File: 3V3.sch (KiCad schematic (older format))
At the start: 1 part, among them SW4 SW_SP3T

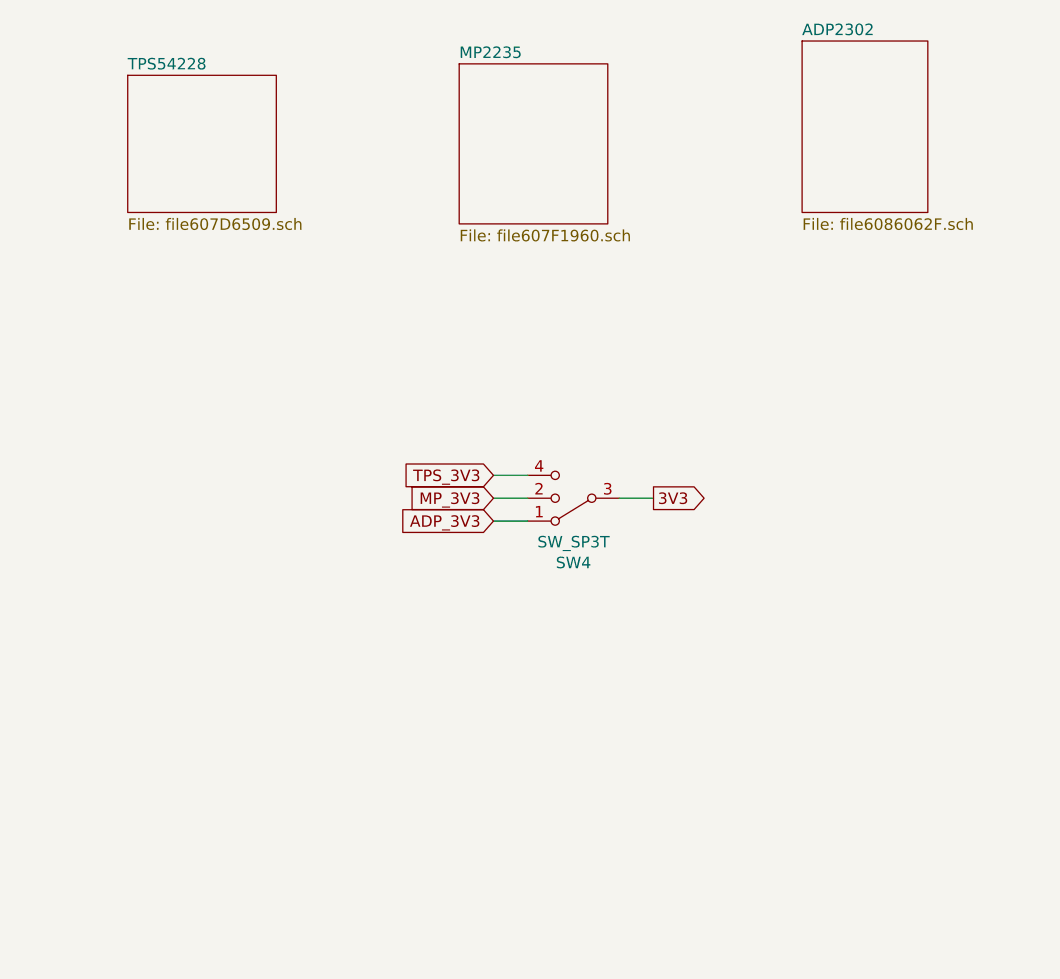
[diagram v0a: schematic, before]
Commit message: full schematic, version 1.0
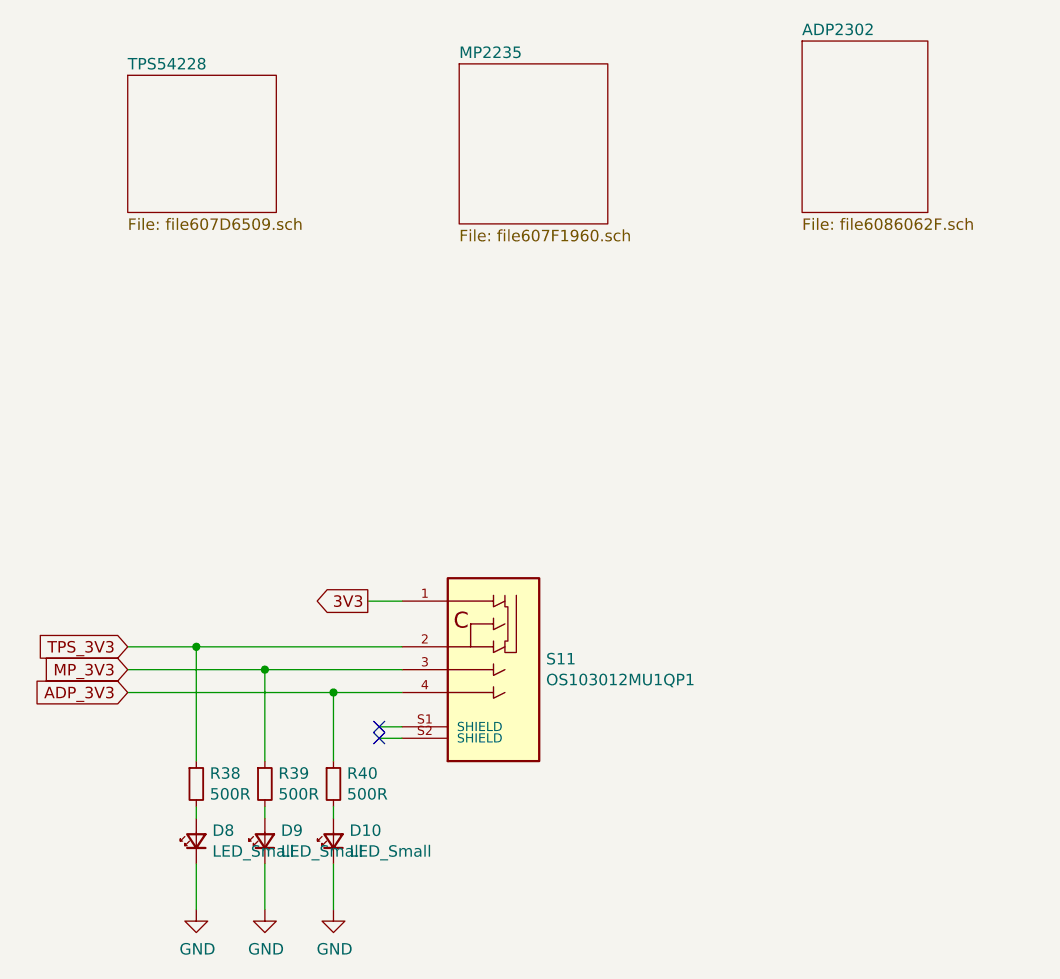
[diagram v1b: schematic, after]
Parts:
- removed SW4: SW_SP3T, symbol Switch:SW_SP3T
- added D10, D8, D9: LED_Small, Diode_SMD:D_0603_1608Metric_Pad1.05x0.95mm_HandSolder, symbol Device:LED_Small
- added R38, R39, R40: 500R, Resistor_SMD:R_0805_2012Metric_Pad1.20x1.40mm_HandSolder, symbol Device:R_Small
- added S11: OS103012MU1QP1, EIPP:SW_OS103012MU1QP1, symbol EIPP_LIBRARY:OS103012MU1QP1
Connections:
- net 3V3: now also S11.1
- net ADP_3V3: now also R40.1, S11.4
- net MP_3V3: now also R39.1, S11.3
- net TPS_3V3: now also R38.1, S11.2
- new net: D8.2 (A), R38.2
- new net: D9.2 (A), R39.2
- new net: D10.2 (A), R40.2
- new net GND: D10.1 (K), D8.1 (K), D9.1 (K)
- no-connect marks 0 -> 2
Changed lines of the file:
@@
 $Descr A4 11693 8268
 encoding utf-8
-Sheet 2 10
+Sheet 2 15
 Title ""
 Date ""
@@
 F1 "file6086062F.sch" 50
 $EndSheet
-Text GLabel 3650 3450 0    50   Input ~ 0
+Text GLabel 2050 4200 0    50   Input ~ 0
 TPS_3V3
-Wire Wire Line
-	3650 3450 3800 3450
-Text GLabel 3650 3550 0    50   Input ~ 0
+Text GLabel 2050 4300 0    50   Input ~ 0
 MP_3V3
-Text GLabel 3650 3650 0    50   Input ~ 0
+Text GLabel 2050 4400 0    50   Input ~ 0
 ADP_3V3
 Wire Wire Line
-	3800 3650 3650 3650
-Wire Wire Line
-	4200 3550 4350 3550
-Text GLabel 4350 3550 2    50   Output ~ 0
+	3250 4000 3100 4000
+Text GLabel 3100 4000 0    50   Output ~ 0
 3V3
 $Comp
-L Switch:SW_SP3T SW4
-U 1 1 608026A5
-P 4000 3550
-F 0 "SW4" H 4000 3833 50  0000 C CNN
-F 1 "SW_SP3T" H 4000 3742 50  0000 C CNN
-F 2 "" H 3375 3725 50  0001 C CNN
-F 3 "~" H 3375 3725 50  0001 C CNN
-	1    4000 3550
-	-1   0    0    1
-$EndComp
-Wire Wire Line
-	3650 3550 3800 3550
+L EIPP_LIBRARY:OS103012MU1QP1 S11
+U 1 1 608F895B
+P 3650 4300
+F 0 "S11" H 3880 4346 50  0000 L CNN
+F 1 "OS103012MU1QP1" H 3880 4255 50  0000 L CNN
+F 2 "EIPP:SW_OS103012MU1QP1" H 3650 4300 50  0001 L BNN
+F 3 "" H 3650 4300 50  0001 L BNN
+F 4 "9.2 mm" H 3650 4300 50  0001 L BNN "MAXIMUM_PACKAGE_HEIGHT"
+F 5 "C and K Switches" H 3650 4300 50  0001 L BNN "MANUFACTURER"
+F 6 "Manufacturer Recommendations" H 3650 4300 50  0001 L BNN "STANDARD"
+F 7 "8 Aug 17" H 3650 4300 50  0001 L BNN "PARTREV"
+	1    3650 4300
+	1    0    0    -1
+$EndComp
+Wire Wire Line
+	3250 4550 3150 4550
+Wire Wire Line
+	3150 4600 3250 4600
+NoConn ~ 3150 4550
+NoConn ~ 3150 4600
+$Comp
+L Device:LED_Small D?
+U 1 1 6082CA23
+P 2350 5050
+AR Path="/60925CA4/6082CA23" Ref="D?"  Part="1"
+AR Path="/607D64D2/6082CA23" Ref="D8"  Part="1"
+F 0 "D8" V 2396 4980 50  0000 R CNN
+F 1 "LED_Small" V 2305 4980 50  0000 R CNN
+F 2 "Diode_SMD:D_0603_1608Metric_Pad1.05x0.95mm_HandSolder" V 2350 5050 50  0001 C CNN
+F 3 "~" V 2350 5050 50  0001 C CNN
+	1    2350 5050
+	0    -1   -1   0
+$EndComp
+$Comp
+L Device:R_Small R?
+U 1 1 6082CA29
+P 2350 4800
+AR Path="/60925CA4/6082CA29" Ref="R?"  Part="1"
+AR Path="/607D64D2/6082CA29" Ref="R38"  Part="1"
+F 0 "R38" H 2409 4846 50  0000 L CNN
+F 1 "500R" H 2409 4755 50  0000 L CNN
+F 2 "Resistor_SMD:R_0805_2012Metric_Pad1.20x1.40mm_HandSolder" H 2350 4800 50  0001 C CNN
+F 3 "~" H 2350 4800 50  0001 C CNN
+	1    2350 4800
+	1    0    0    -1
+$EndComp
+Wire Wire Line
+	2350 4950 2350 4900
+Wire Wire Line
+	2350 4700 2350 4200
+Wire Wire Line
+	2350 5150 2350 5350
+$Comp
+L power:GND #PWR?
+U 1 1 6082CA32
+P 2350 5350
+AR Path="/60925CA4/6082CA32" Ref="#PWR?"  Part="1"
+AR Path="/607D64D2/6082CA32" Ref="#PWR059"  Part="1"
+F 0 "#PWR059" H 2350 5100 50  0001 C CNN
+F 1 "GND" H 2355 5177 50  0000 C CNN
+F 2 "" H 2350 5350 50  0001 C CNN
+F 3 "" H 2350 5350 50  0001 C CNN
+	1    2350 5350
+	1    0    0    -1
+$EndComp
+$Comp
+L Device:LED_Small D?
+U 1 1 6082CA38
+P 2650 5050
+AR Path="/60925CA4/6082CA38" Ref="D?"  Part="1"
+AR Path="/607D64D2/6082CA38" Ref="D9"  Part="1"
+F 0 "D9" V 2696 4980 50  0000 R CNN
+F 1 "LED_Small" V 2605 4980 50  0000 R CNN
+F 2 "Diode_SMD:D_0603_1608Metric_Pad1.05x0.95mm_HandSolder" V 2650 5050 50  0001 C CNN
+F 3 "~" V 2650 5050 50  0001 C CNN
+	1    2650 5050
+	0    -1   -1   0
+$EndComp
+$Comp
+L Device:R_Small R?
+U 1 1 6082CA3E
+P 2650 4800
+AR Path="/60925CA4/6082CA3E" Ref="R?"  Part="1"
+AR Path="/607D64D2/6082CA3E" Ref="R39"  Part="1"
+F 0 "R39" H 2709 4846 50  0000 L CNN
+F 1 "500R" H 2709 4755 50  0000 L CNN
+F 2 "Resistor_SMD:R_0805_2012Metric_Pad1.20x1.40mm_HandSolder" H 2650 4800 50  0001 C CNN
+F 3 "~" H 2650 4800 50  0001 C CNN
+	1    2650 4800
+	1    0    0    -1
+$EndComp
+Wire Wire Line
+	2650 4950 2650 4900
+Wire Wire Line
+	2650 5150 2650 5350
+$Comp
+L power:GND #PWR?
+U 1 1 6082CA46
+P 2650 5350
+AR Path="/60925CA4/6082CA46" Ref="#PWR?"  Part="1"
+AR Path="/607D64D2/6082CA46" Ref="#PWR060"  Part="1"
+F 0 "#PWR060" H 2650 5100 50  0001 C CNN
+F 1 "GND" H 2655 5177 50  0000 C CNN
+F 2 "" H 2650 5350 50  0001 C CNN
+F 3 "" H 2650 5350 50  0001 C CNN
+	1    2650 5350
+	1    0    0    -1
+$EndComp
+$Comp
+L Device:LED_Small D?
+U 1 1 6082CA4C
+P 2950 5050
+AR Path="/60925CA4/6082CA4C" Ref="D?"  Part="1"
+AR Path="/607D64D2/6082CA4C" Ref="D10"  Part="1"
+F 0 "D10" V 2996 4980 50  0000 R CNN
+F 1 "LED_Small" V 2905 4980 50  0000 R CNN
+F 2 "Diode_SMD:D_0603_1608Metric_Pad1.05x0.95mm_HandSolder" V 2950 5050 50  0001 C CNN
+F 3 "~" V 2950 5050 50  0001 C CNN
+	1    2950 5050
+	0    -1   -1   0
+$EndComp
+$Comp
+L Device:R_Small R?
+U 1 1 6082CA52
+P 2950 4800
+AR Path="/60925CA4/6082CA52" Ref="R?"  Part="1"
+AR Path="/607D64D2/6082CA52" Ref="R40"  Part="1"
+F 0 "R40" H 3009 4846 50  0000 L CNN
+F 1 "500R" H 3009 4755 50  0000 L CNN
+F 2 "Resistor_SMD:R_0805_2012Metric_Pad1.20x1.40mm_HandSolder" H 2950 4800 50  0001 C CNN
+F 3 "~" H 2950 4800 50  0001 C CNN
+	1    2950 4800
+	1    0    0    -1
+$EndComp
+Wire Wire Line
+	2950 4950 2950 4900
+Wire Wire Line
+	2950 5150 2950 5350
+$Comp
+L power:GND #PWR?
+U 1 1 6082CA5A
+P 2950 5350
+AR Path="/60925CA4/6082CA5A" Ref="#PWR?"  Part="1"
+AR Path="/607D64D2/6082CA5A" Ref="#PWR061"  Part="1"
+F 0 "#PWR061" H 2950 5100 50  0001 C CNN
+F 1 "GND" H 2955 5177 50  0000 C CNN
+F 2 "" H 2950 5350 50  0001 C CNN
+F 3 "" H 2950 5350 50  0001 C CNN
+	1    2950 5350
+	1    0    0    -1
+$EndComp
+Wire Wire Line
+	2650 4300 2650 4700
+Wire Wire Line
+	2950 4400 2950 4700
+Wire Wire Line
+	2950 4400 3250 4400
+Wire Wire Line
+	2950 4400 2050 4400
+Connection ~ 2950 4400
+Wire Wire Line
+	2050 4300 2650 4300
+Wire Wire Line
+	2650 4300 3250 4300
+Connection ~ 2650 4300
+Wire Wire Line
+	2350 4200 3250 4200
+Wire Wire Line
+	2350 4200 2050 4200
+Connection ~ 2350 4200
 $EndSCHEMATC
